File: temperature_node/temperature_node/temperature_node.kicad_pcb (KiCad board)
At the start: 4 copper layers, 23 x 24.5 mm, 34 parts, among them CN1 UART, J1 USB_C_Receptacle_USB2.0_16P, J2 S2B-PH-K-S, U1 SHT40-AD1B-R3, U2 MCP73831-2-OT, U3 MIC5504-3.3YM5, U4 ESP32-C3-WROOM-02

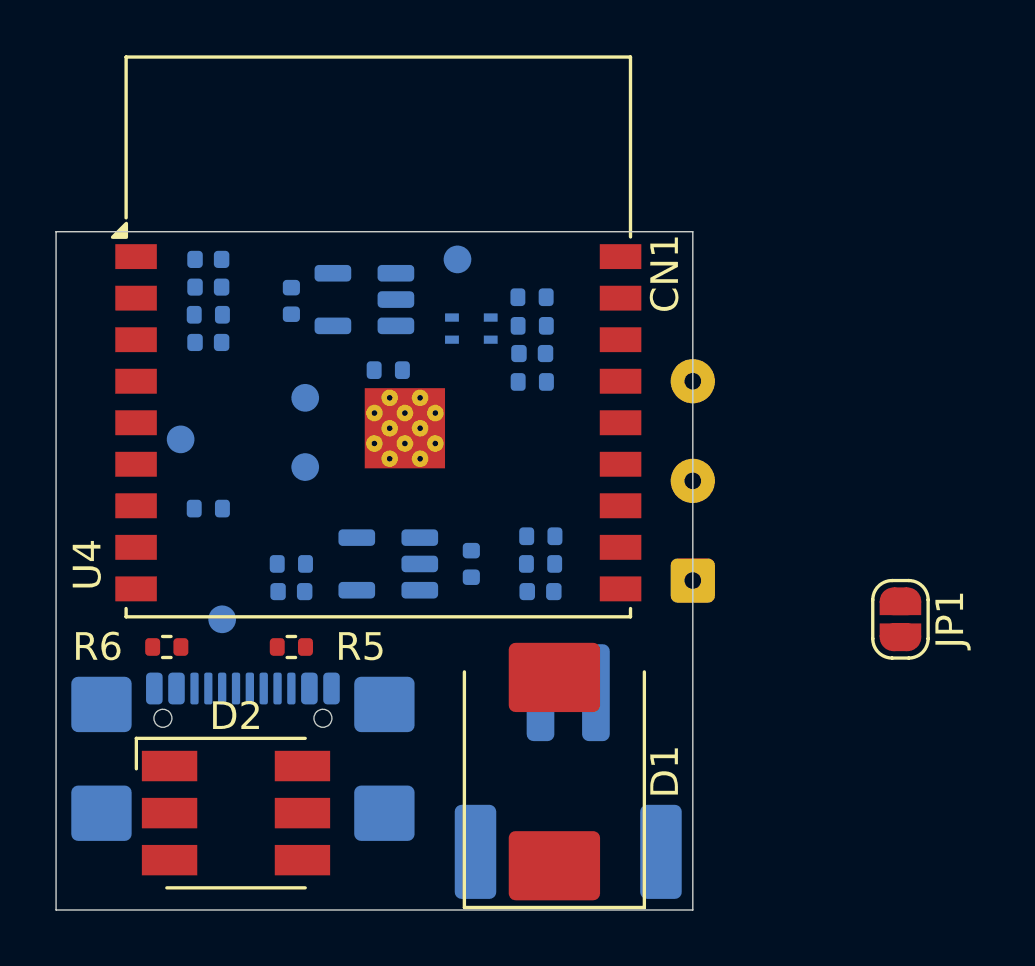
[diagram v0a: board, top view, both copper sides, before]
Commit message: Placement pre routing
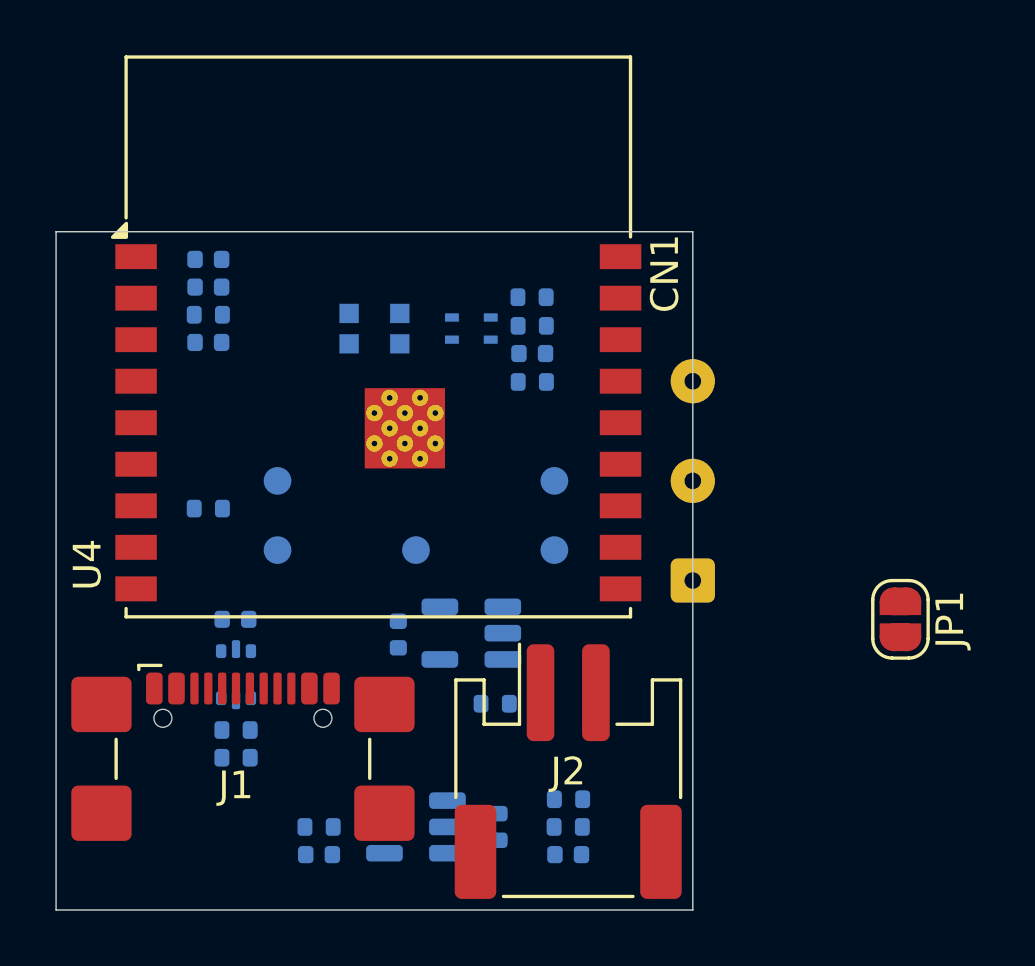
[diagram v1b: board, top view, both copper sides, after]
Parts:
- removed D1: 1.5SMC6.8CA, Diode_SMD:D_SMC
- removed D2: APA102, LED_SMD:LED_RGB_5050-6
- added C9: 100n, Capacitor_SMD:C_0402_1005Metric, B.Cu at (127.5, 94.0)
- added D3: WS2812B-2020, LED_SMD:LED_WS2812B-2020_PLCC4_2.0x2.0mm, B.Cu at (132.5, 83.5)
- added U6: USBLC6-2P6, Package_TO_SOT_SMD:SOT-666, B.Cu at (127.5, 96.0)
- J1, J2: moved to F.Cu
- R5, R6: moved to B.Cu
- moved TP5 13.6 mm to (139.0, 89.0)
- moved C5 12.7 mm to (133.4, 94.5)
- moved R4 12.7 mm to (136.9, 97.0)
- moved U3 12.7 mm to (136.0, 94.5)
- moved TP3 10.3 mm to (129.0, 89.0)
- moved C2 9.55 mm to (130.5, 102.5)
- moved C3 9.55 mm to (139.5, 102.5)
- moved C4 9.55 mm to (137.0, 101.5)
- moved R11 9.55 mm to (139.5, 101.5)
- moved R12 9.55 mm to (139.5, 100.5)
- moved R3 9.55 mm to (130.5, 101.5)
- moved U2 9.55 mm to (134.0, 101.5)
- moved TP2 9.49 mm to (139.0, 91.5)
- moved TP4 6.80 mm to (134.0, 91.5)
- moved R6 4.72 mm to (127.5, 99.0)
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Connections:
- J1 pad A6: /D+ -> Net-(J1-D+-PadA6)
- J1 pad A7: /D- -> Net-(J1-D--PadA7)
- J1 pad B6: /D+ -> Net-(J1-D+-PadA6)
- J1 pad B7: /D- -> Net-(J1-D--PadA7)
- U4 pad 4: /LED_CI -> /GPIO5
